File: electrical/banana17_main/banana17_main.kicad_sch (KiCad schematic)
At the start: 26 parts, among them J1 78171-0004, U1 RP2040, U2 NCP1117-3.3_SOT223, U3 ssd1306_128x32, U4 W25Q128JVS, Y1 ABMB-272-T3

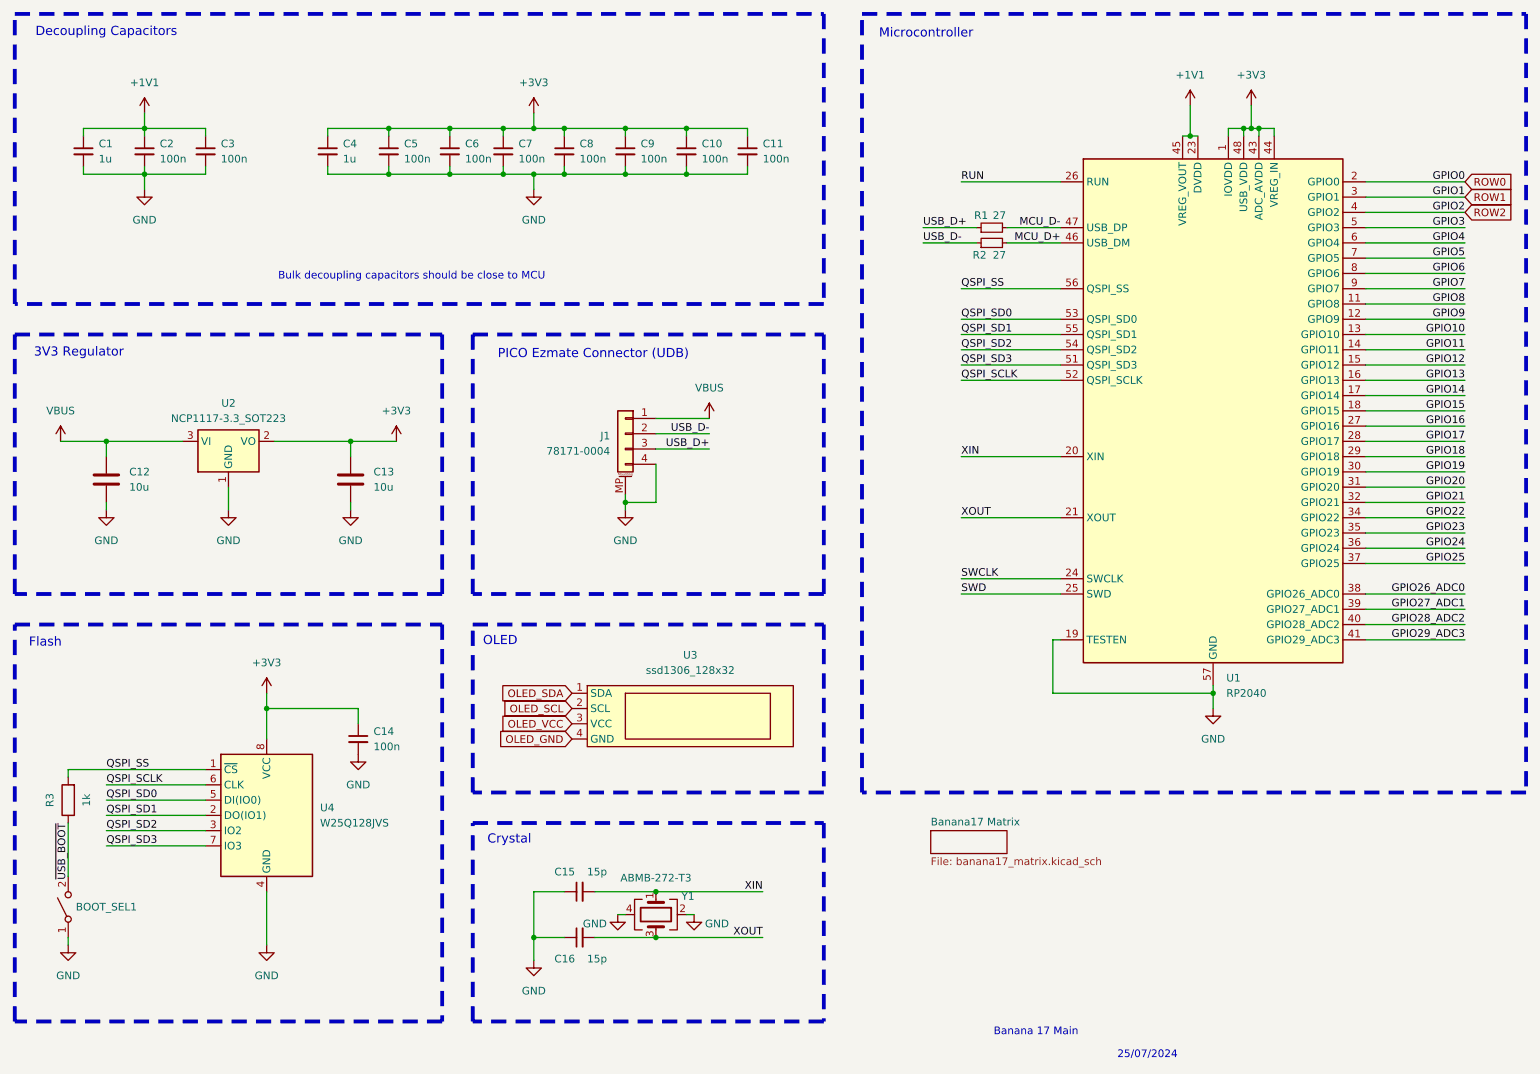
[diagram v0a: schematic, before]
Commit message: Incorporated USB C connector. Shrunk overall design.
Incorporated USB C connector. Shrunk overall design.
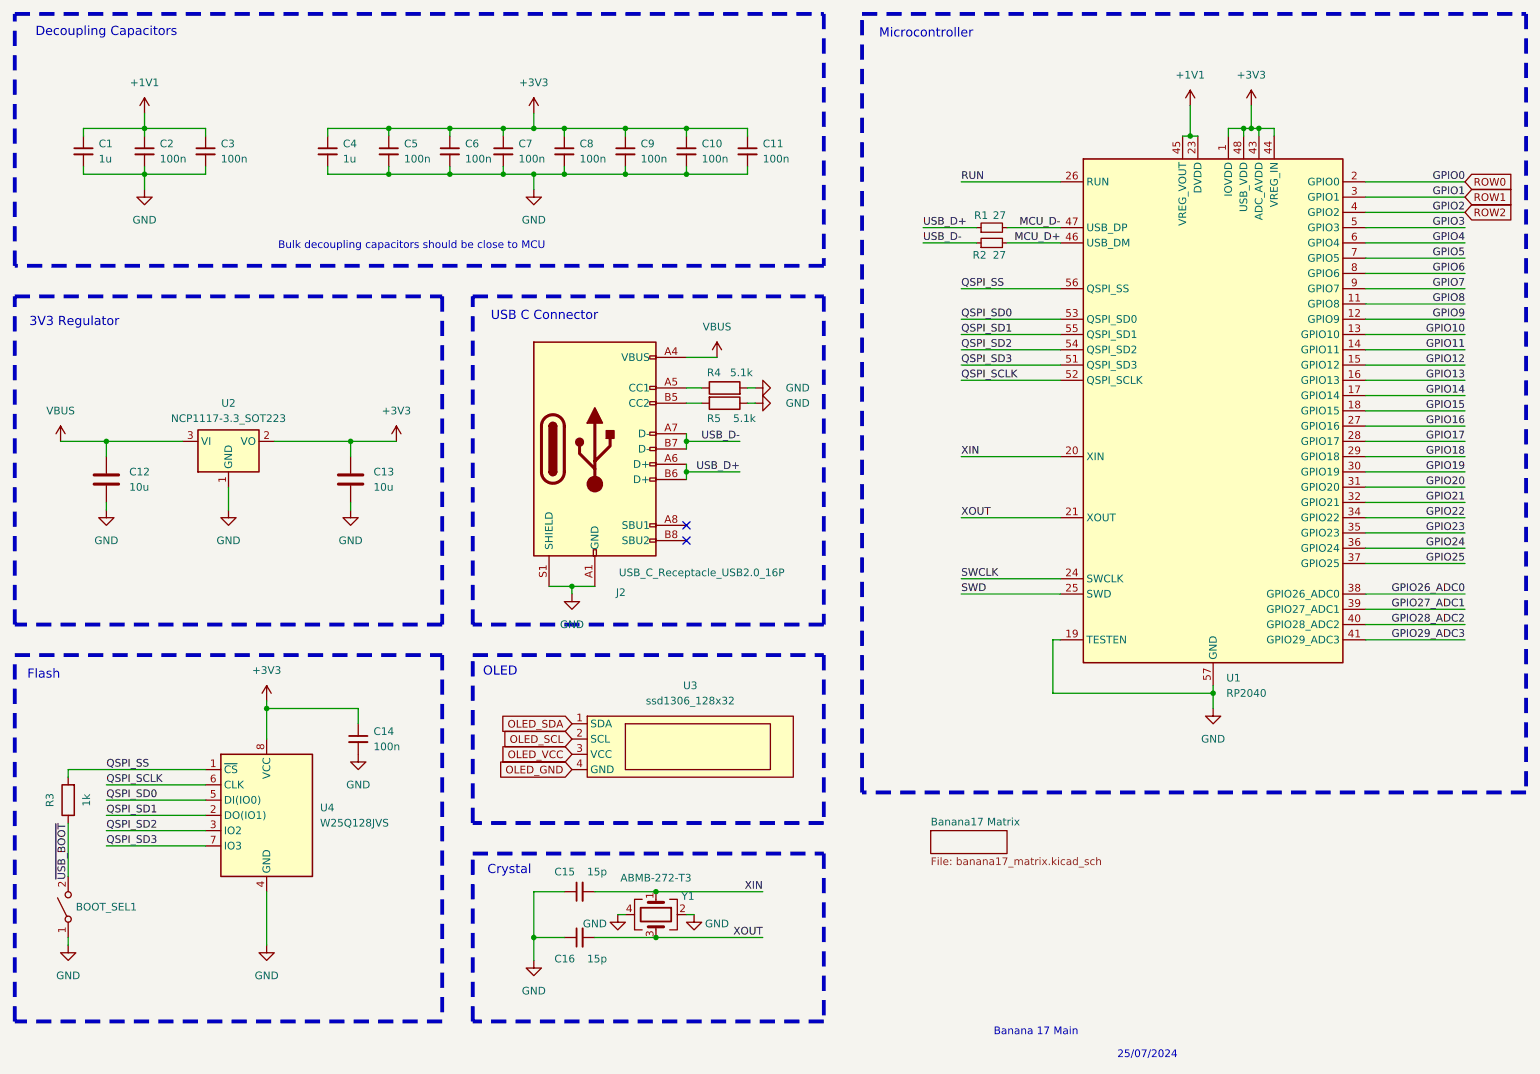
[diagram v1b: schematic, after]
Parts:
- removed J1: 78171-0004, Connector_Molex:Molex_Pico-EZmate_78171-0004_1x04-1MP_P1.20mm_Vertical, symbol Connector_Generic_MountingPin:Conn_01x04_MountingPin
- added J2: USB_C_Receptacle_USB2.0_16P, locallib:HRO-TYPE-C-31-M-12-Assembly, symbol Connector:USB_C_Receptacle_USB2.0_16P
- added R4, R5: 5.1k, Resistor_SMD:R_0402_1005Metric_Pad0.72x0.64mm_HandSolder, symbol Device:R
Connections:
- net GND: now also J2.A1 (GND), J2.A12 (GND), J2.B1 (GND), J2.B12 (GND), J2.S1 (SHIELD), R4.2, R5.1
- net USB_D+: now also J2.A6 (D+), J2.B6 (D+)
- net USB_D-: now also J2.A7 (D-), J2.B7 (D-)
- net VBUS: now also J2.A4 (VBUS), J2.A9 (VBUS), J2.B4 (VBUS), J2.B9 (VBUS)
- new net: J2.B5 (CC2), R5.2
- new net: J2.A5 (CC1), R4.1
- no-connect marks 0 -> 2
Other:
- note added: "USB C Connector"
- note removed: "PICO Ezmate Connector (UDB)"
- moved on the sheet: U3
